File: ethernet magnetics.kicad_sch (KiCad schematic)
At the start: 3 parts

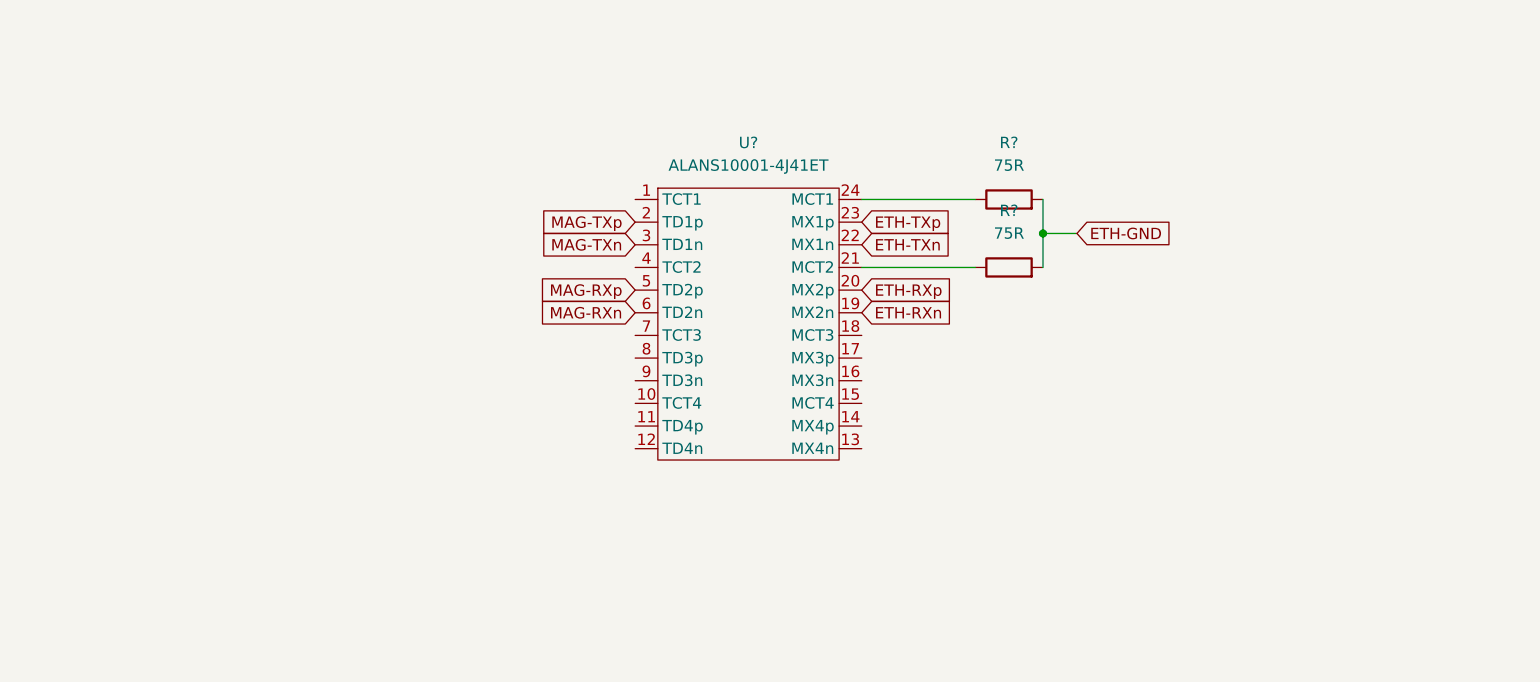
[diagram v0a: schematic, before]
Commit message: wired phy controller
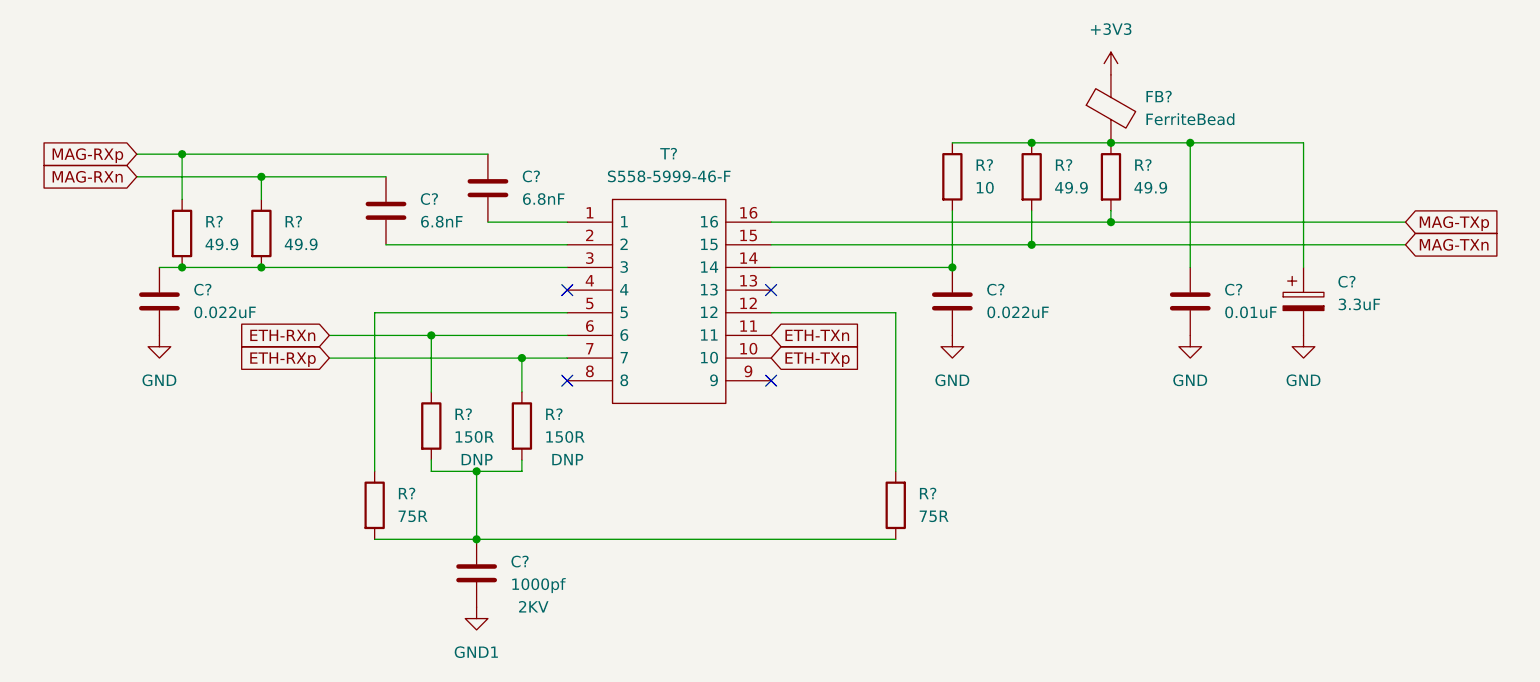
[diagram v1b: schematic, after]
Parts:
- removed U?: ALANS10001-4J41ET, symbol local_library:ALANS10001-4J41ET
- added C? (x2): 6.8nF, symbol Device:C
- added C? (x2): 0.022uF, symbol Device:C
- added C?: 0.01uF, symbol Device:C
- added C?: 3.3uF, symbol Device:C_Polarized
- added C?: 1000pf, symbol Device:C
- added FB?: FerriteBead, symbol Device:FerriteBead
- added R? (x4): 49.9, symbol Device:R
- added R? (x2): 150R, symbol Device:R
- added R?: 10, symbol Device:R
- added T?: S558-5999-46-F, SOP254P1270X597-16N, symbol SamacSys_Parts:S558-5999-46-F
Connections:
- net ETH-RXn: now also R?.1, T?.6
- net ETH-RXp: now also R?.1, T?.7
- net ETH-TXn: now also T?.11
- net ETH-TXp: now also T?.10
- net MAG-RXn: now also C?.1, R?.1
- net MAG-RXp: now also C?.1, R?.1
- net MAG-TXn: now also R?.2, T?.15
- net MAG-TXp: now also R?.2, T?.16
- net at R?.1: now also T?.5
- net at R?.1: now also R?.2, C?.1, R?.2, R?.2
- net ETH-GND: no longer names the net of R?.2
- net ETH-GND: now also T?.12; no longer R?.2
- new net: C?.2, T?.1
- new net: C?.1, R?.2, R?.2, T?.3
- new net: C?.1, C?.1, FB?.2, R?.1, R?.1, R?.1
- new net: C?.1, R?.2, T?.14
- new net: C?.2, T?.2
- new net +3V3: FB?.1
- new net GND: C?.2, C?.2, C?.2, C?.2
- new net GND1: C?.2
- no-connect marks 0 -> 4
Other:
- moved on the sheet: R?
